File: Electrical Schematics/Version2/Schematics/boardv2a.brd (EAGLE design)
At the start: 188.8 x 159.4 mm, 559 parts, among them IC1 MCP41HVX1ST, IC2 ADUM4160BRW, IC3 SE555D, IC5 74LVC1G04DBV, IC6 74LVC1G04DBV, IC7 4030D, K1 G5V-2, Q1 IRLML2060TRPBFBSS123LT1G, Q10 IRLML2060TRPBFBSS123LT1G, Q11 IRLML2060TRPBFBSS123LT1G, Q13 IRLML2060TRPBFBSS123LT1G, Q14 IRLML2060TRPBFBSS123LT1G, Q15 IRLML2060TRPBFBSS123LT1G, Q16 IRLML2060TRPBFBSS123LT1G, Q17 IRLML2060TRPBFBSS123LT1G, Q18 BSP170P, Q19 IRLML2060TRPBFBSS123LT1G, Q2 IRLML2060TRPBFBSS123LT1G, Q3 IRLML2060TRPBFBSS123LT1G, Q4 BSP170P, Q5 IRLML2060TRPBFBSS123LT1G, Q6 IRLML2060TRPBFBSS123LT1G, Q7 ASFL1, Q8 IRLML2060TRPBFBSS123LT1G, Q9 IRLML2060TRPBFBSS123LT1G, U1 CP2130-GM, U10 SN65HVDA100-Q1_D_8, U11 ADUM3442CRWZ, U12 ADUM3442CRWZ, U13 ADUM3442CRWZ, U14 ADUM3442CRWZ, U15 ADUM3442CRWZ, U16 ADUM3442CRWZ, U17 ADUM3442CRWZ, U18 LM1085_KTT_3, U19 ADUM3442CRWZ, U2 TMS570LS0432_PZ_100, U20 ADUM3442CRWZ, U3 LM1085_KTT_3, U4 LM1085_KTT_3, U5 LM1084_KTT_3, U6 TPS3514_D_14, U7 LM1085_KTT_3, U9 ADUM3442CRWZ, X4 5566-4

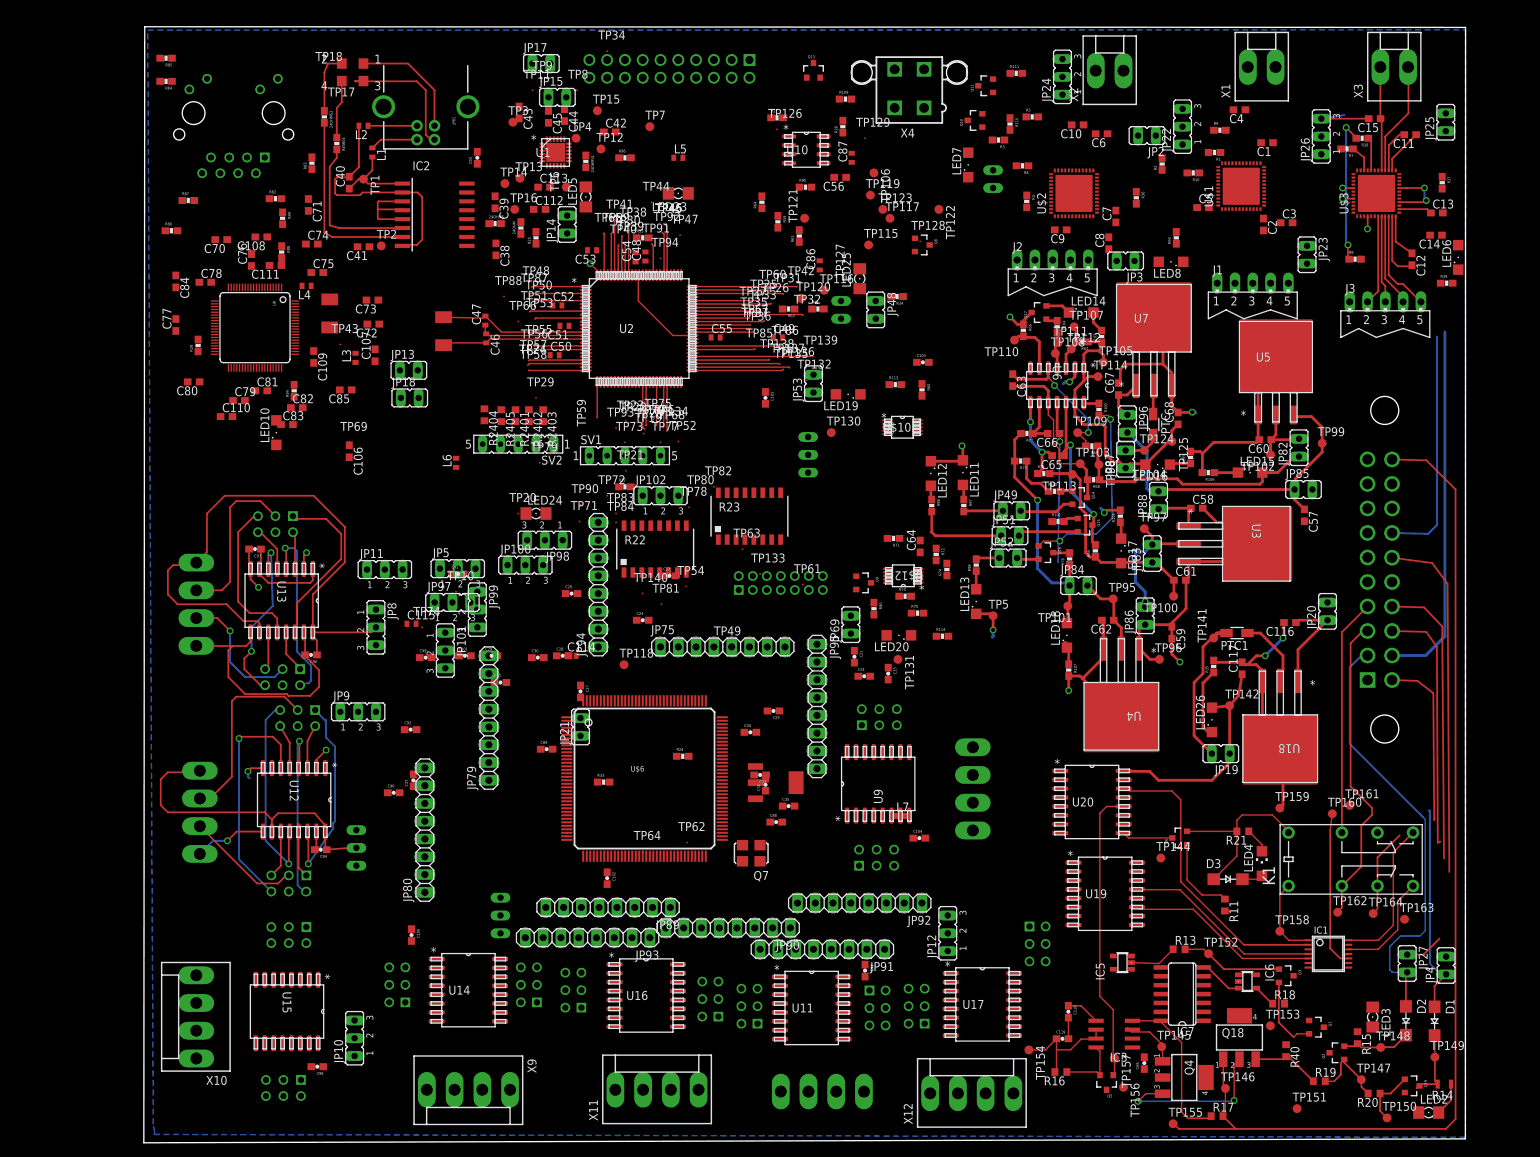
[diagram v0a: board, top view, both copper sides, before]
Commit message: did some lagit routing
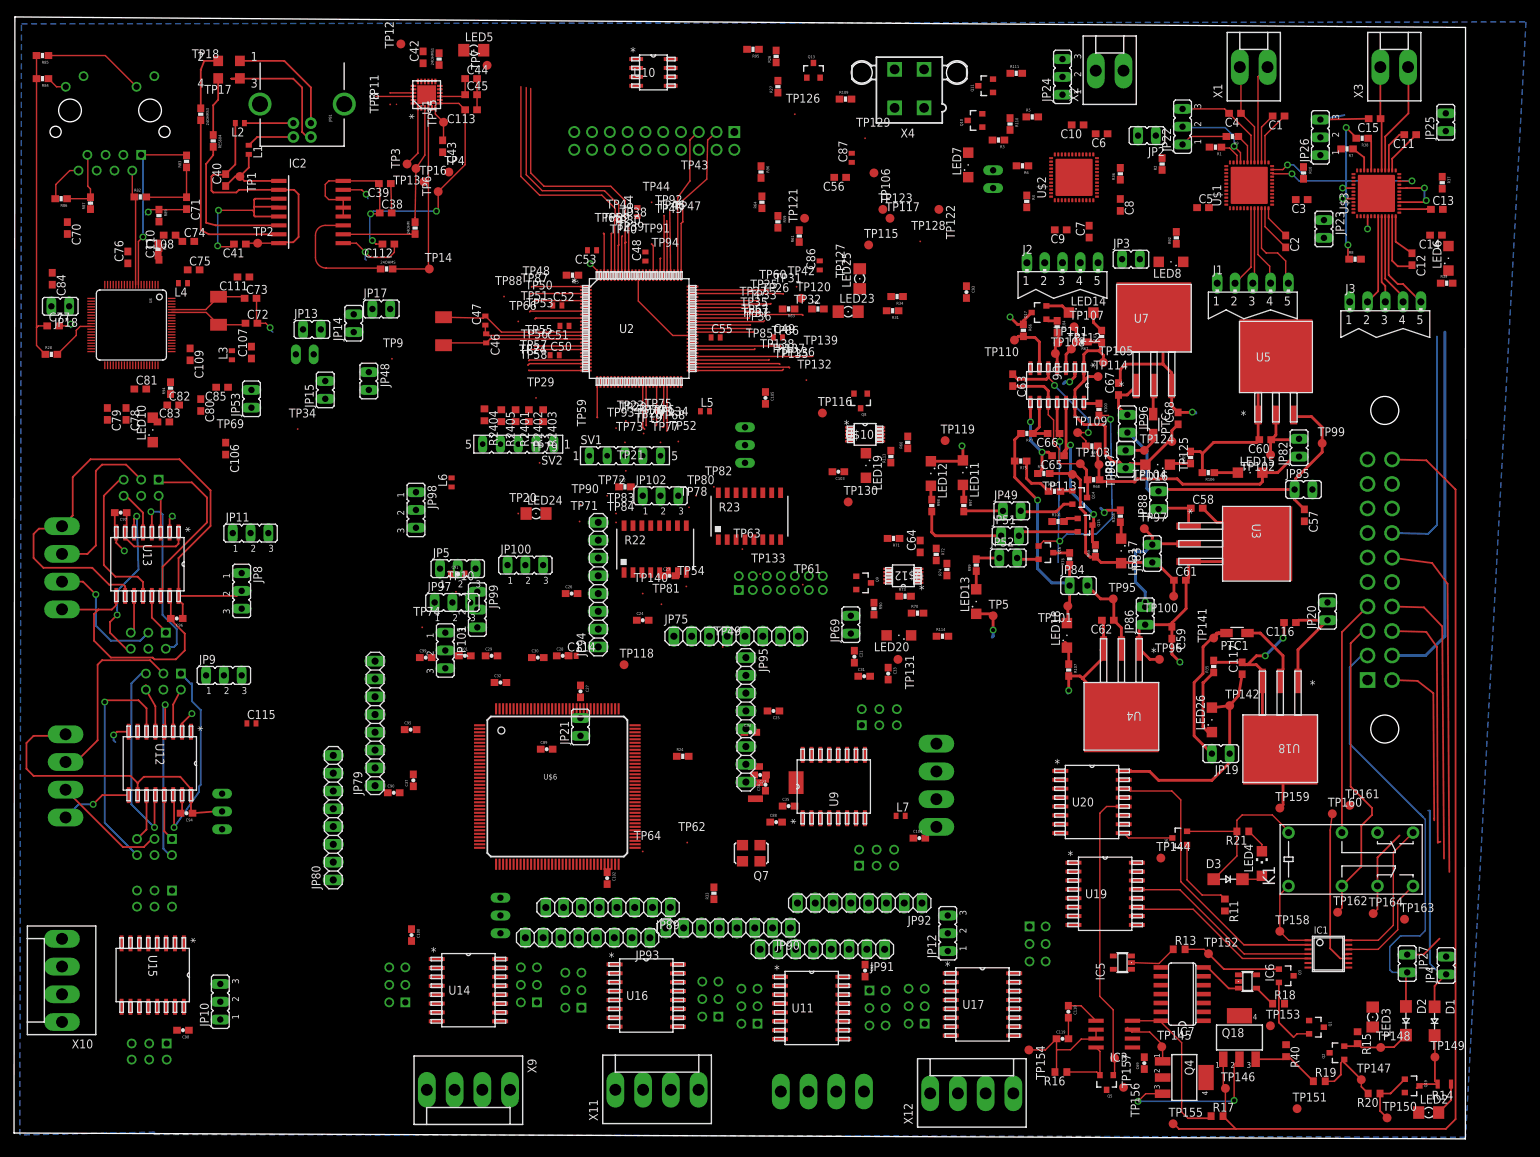
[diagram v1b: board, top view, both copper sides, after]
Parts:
- moved JP53 80.3 mm to (17.8, 49.4)
- moved JP16 76.8 mm to (25.4, 55.8), turned to 90 degrees
- moved JP48 73.1 mm to (34.5, 51.9)
- moved C93 72.4 mm to (119.9, 64.6), turned to 270 degrees
- moved TP34 69.8 mm to (24.4, 45.1)
- moved TP43 55.1 mm to (80.4, 80.5)
- moved JP15 53.3 mm to (28.3, 50.7), turned to 0 degrees
- moved JP18 51.6 mm to (-9.53, 62.6), turned to 90 degrees
- moved TP9 45.0 mm to (37.8, 55.1)
- moved JP17 41.8 mm to (36.3, 62.2)
- moved R31 37.2 mm to (109.3, 62.0), turned to 180 degrees
- moved TP119 36.6 mm to (116.8, 43.4)
- moved L5 36.4 mm to (82.5, 47.6)
- moved JP14 33.6 mm to (32.4, 60.2)
- moved TP12 32.3 mm to (39.1, 100.1), turned to 90 degrees
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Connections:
- net MCU_COMMS_MISO: now also JP14.1
- net MCU_COMMS_SCK: now also JP18.2
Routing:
- net SPIBRIDGE_ISOLATION_VBUS: track 0.00 -> 56.8 mm, vias 0 -> 3
- net GND: track 186.4 -> 240.5 mm, vias 18 -> 23
- net ETHERNET_3.3_J_+: track 0.00 -> 44.8 mm
- net MCU_LIN_EN: track 4.74 -> 38.0 mm
- net MCU__LINRX: track 4.35 -> 37.5 mm
- net MCU_LINTX: track 7.91 -> 37.7 mm
- net SPIBRIDGE_ISOLATION_D-: track 0.00 -> 28.3 mm
- net 0.1: track 0.00 -> 25.4 mm, vias 0 -> 1
- net MCU_PROG_NTRST: track 0.00 -> 22.6 mm
- net MCU_BATMON_LIN: track 0.00 -> 22.2 mm, vias 0 -> 2
- net MCU_PROG_TDI: track 0.00 -> 21.6 mm
- net MONA_AGND: track 0.00 -> 19.3 mm, vias 0 -> 1
- net N$114: track 0.00 -> 17.7 mm
- net SPIBRIDGE_ISOLATION_D+: track 0.00 -> 16.7 mm
- net N$199: track 0.00 -> 16.5 mm
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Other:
- board size 188.8 x 159.4 mm -> 207.3 x 160.2 mm
